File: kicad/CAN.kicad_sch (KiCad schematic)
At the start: 1 part, among them U6 SN65HVD231

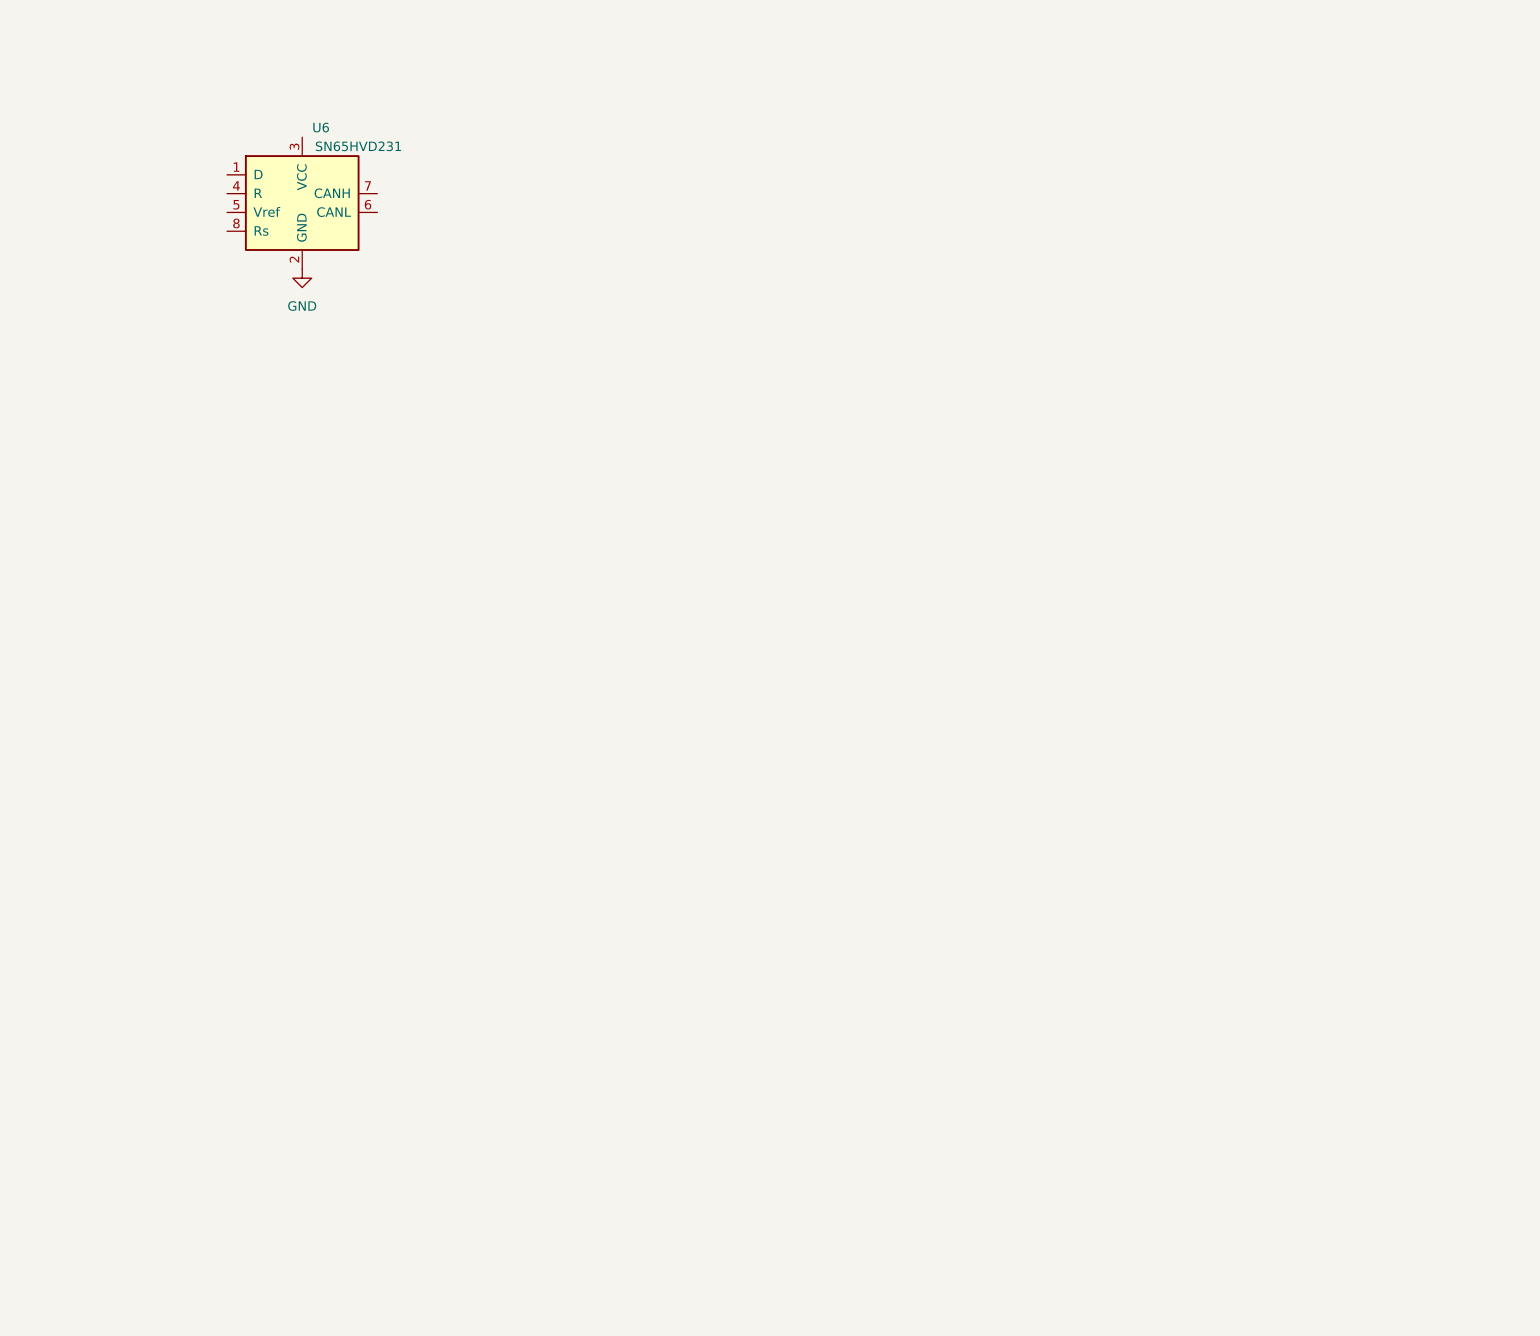
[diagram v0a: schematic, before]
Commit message: WIP
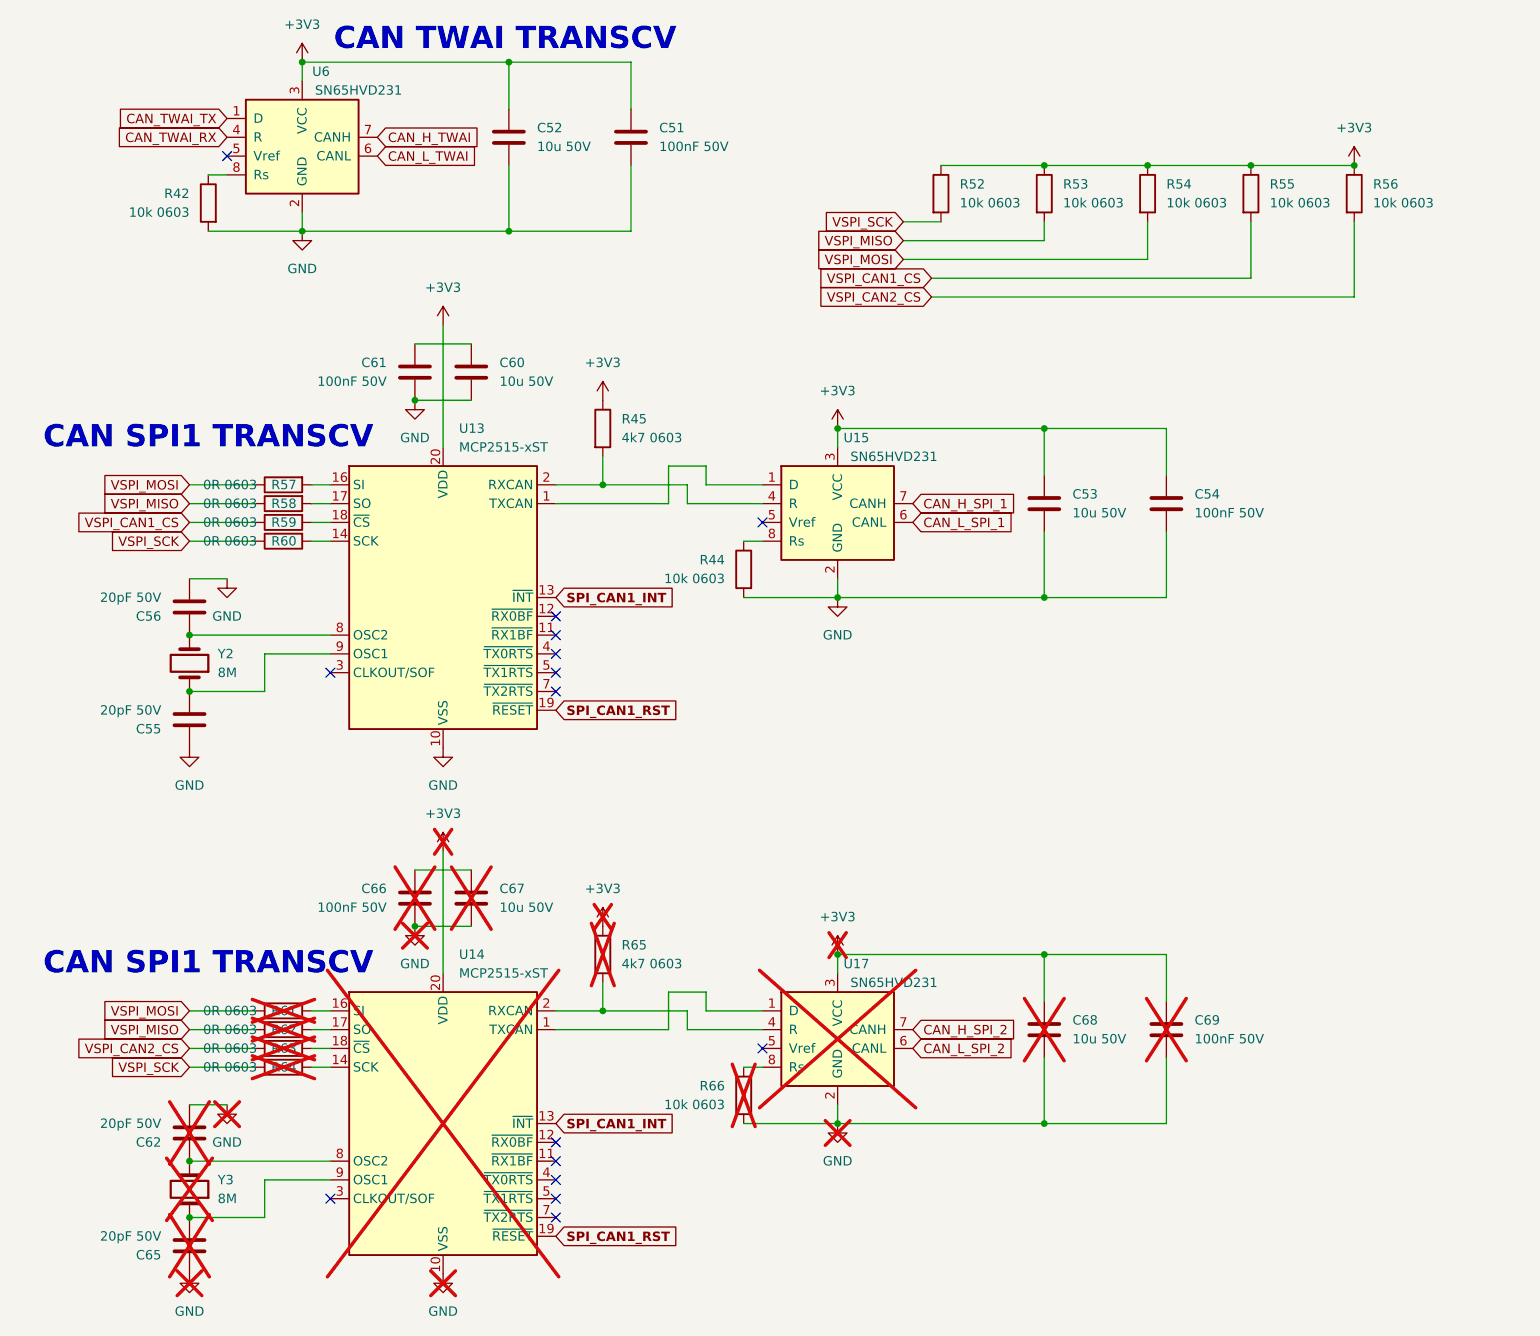
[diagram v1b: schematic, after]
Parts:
- added C51, C54, C61, C66, C69: 100nF 50V, Capacitor_SMD:C_0603_1608Metric, symbol Device:C
- added C52, C53, C60, C67, C68: 10u 50V, Capacitor_SMD:C_1206_3216Metric, symbol Device:C
- added C55, C56, C62, C65: 20pF 50V, Capacitor_SMD:C_0603_1608Metric, symbol Device:C
- added R42, R44, R52, R53, R54, R55, R56, R66: 10k 0603, Resistor_SMD:R_0603_1608Metric, symbol Device:R
- added R45, R65: 4k7 0603, Resistor_SMD:R_0603_1608Metric, symbol Device:R
- added R57, R58, R59, R60, R61, R62, R63, R64: 0R 0603, Resistor_SMD:R_0603_1608Metric, symbol Device:R
- added U13, U14: MCP2515-xST, Package_SO:TSSOP-20_4.4x6.5mm_P0.65mm, symbol Interface_CAN_LIN:MCP2515-xST
- added U15, U17: SN65HVD231, Package_SO:SOIC-8_3.9x4.9mm_P1.27mm, symbol Interface_CAN_LIN:SN65HVD231
- added Y2, Y3: 8M, Crystal:Crystal_HC49-U_Horizontal, symbol Device:Crystal
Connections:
- net GND: now also C51.2, C52.2, C53.2, C54.2, C55.1, C56.2, C60.2, C61.2, C62.2, C65.1, C66.2, C67.2, C68.2, C69.2, R42.2, R44.2, R66.2, U13.10 (VSS), U14.10 (VSS), U15.2 (GND), U17.2 (GND)
- net CAN_TWAI_TX: now reaches U6.1 (D)
- net +3V3: now reaches U6.3 (VCC)
- net +3V3: now also C51.1, C52.1, C53.1, C54.1, C68.1, C69.1, R45.1, R52.1, R53.1, R54.1, R55.1, R56.1, R65.1, U13.20 (VDD), U14.20 (VDD), U15.3 (VCC), U17.3 (VCC)
- net CAN_TWAI_RX: now reaches U6.4 (R)
- net CAN_L_TWAI: now reaches U6.6 (CANL)
- net CAN_H_TWAI: now reaches U6.7 (CANH)
- net at U6.8 (Rs): now also R42.1
- new net: R45.2, U13.2 (RXCAN), U15.4 (R)
- new net: C55.2, U13.9 (OSC1), Y2.1
- new net: R61.2, U14.16 (SI)
- new net: R65.2, U14.2 (RXCAN), U17.4 (R)
- new net: C56.1, U13.8 (OSC2), Y2.2
- new net: C66.1, C67.1
- new net: R44.1, U15.8 (Rs)
- new net: U13.1 (TXCAN), U15.1 (D)
- new net: R60.2, U13.14 (SCK)
- new net: R57.2, U13.16 (SI)
- new net: R58.2, U13.17 (SO)
- new net: R59.2, U13.18 (~{CS})
- new net: R66.1, U17.8 (Rs)
- new net: U14.1 (TXCAN), U17.1 (D)
- new net: R64.2, U14.14 (SCK)
- new net: R62.2, U14.17 (SO)
- new net: R63.2, U14.18 (~{CS})
- new net: C62.1, U14.8 (OSC2), Y3.2
- new net: C65.2, U14.9 (OSC1), Y3.1
- new net: C60.1, C61.1
- new net CAN_H_SPI_1: U15.7 (CANH)
- new net CAN_H_SPI_2: U17.7 (CANH)
- new net CAN_L_SPI_1: U15.6 (CANL)
- new net CAN_L_SPI_2: U17.6 (CANL)
- new net SPI_CAN1_INT: U13.13 (~{INT}), U14.13 (~{INT})
- new net SPI_CAN1_RST: U13.19 (~{RESET}), U14.19 (~{RESET})
- new net VSPI_CAN1_CS: R55.2, R59.1
- new net VSPI_CAN2_CS: R56.2, R63.1
- new net VSPI_MISO: R53.2, R58.1, R62.1
- new net VSPI_MOSI: R54.2, R57.1, R61.1
- new net VSPI_SCK: R52.2, R60.1, R64.1
- no-connect marks 0 -> 15
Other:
- note added: "CAN SPI1 TRANSCV"
- note added: "CAN TWAI TRANSCV"
- moved on the sheet: U6

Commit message: sch done-ish
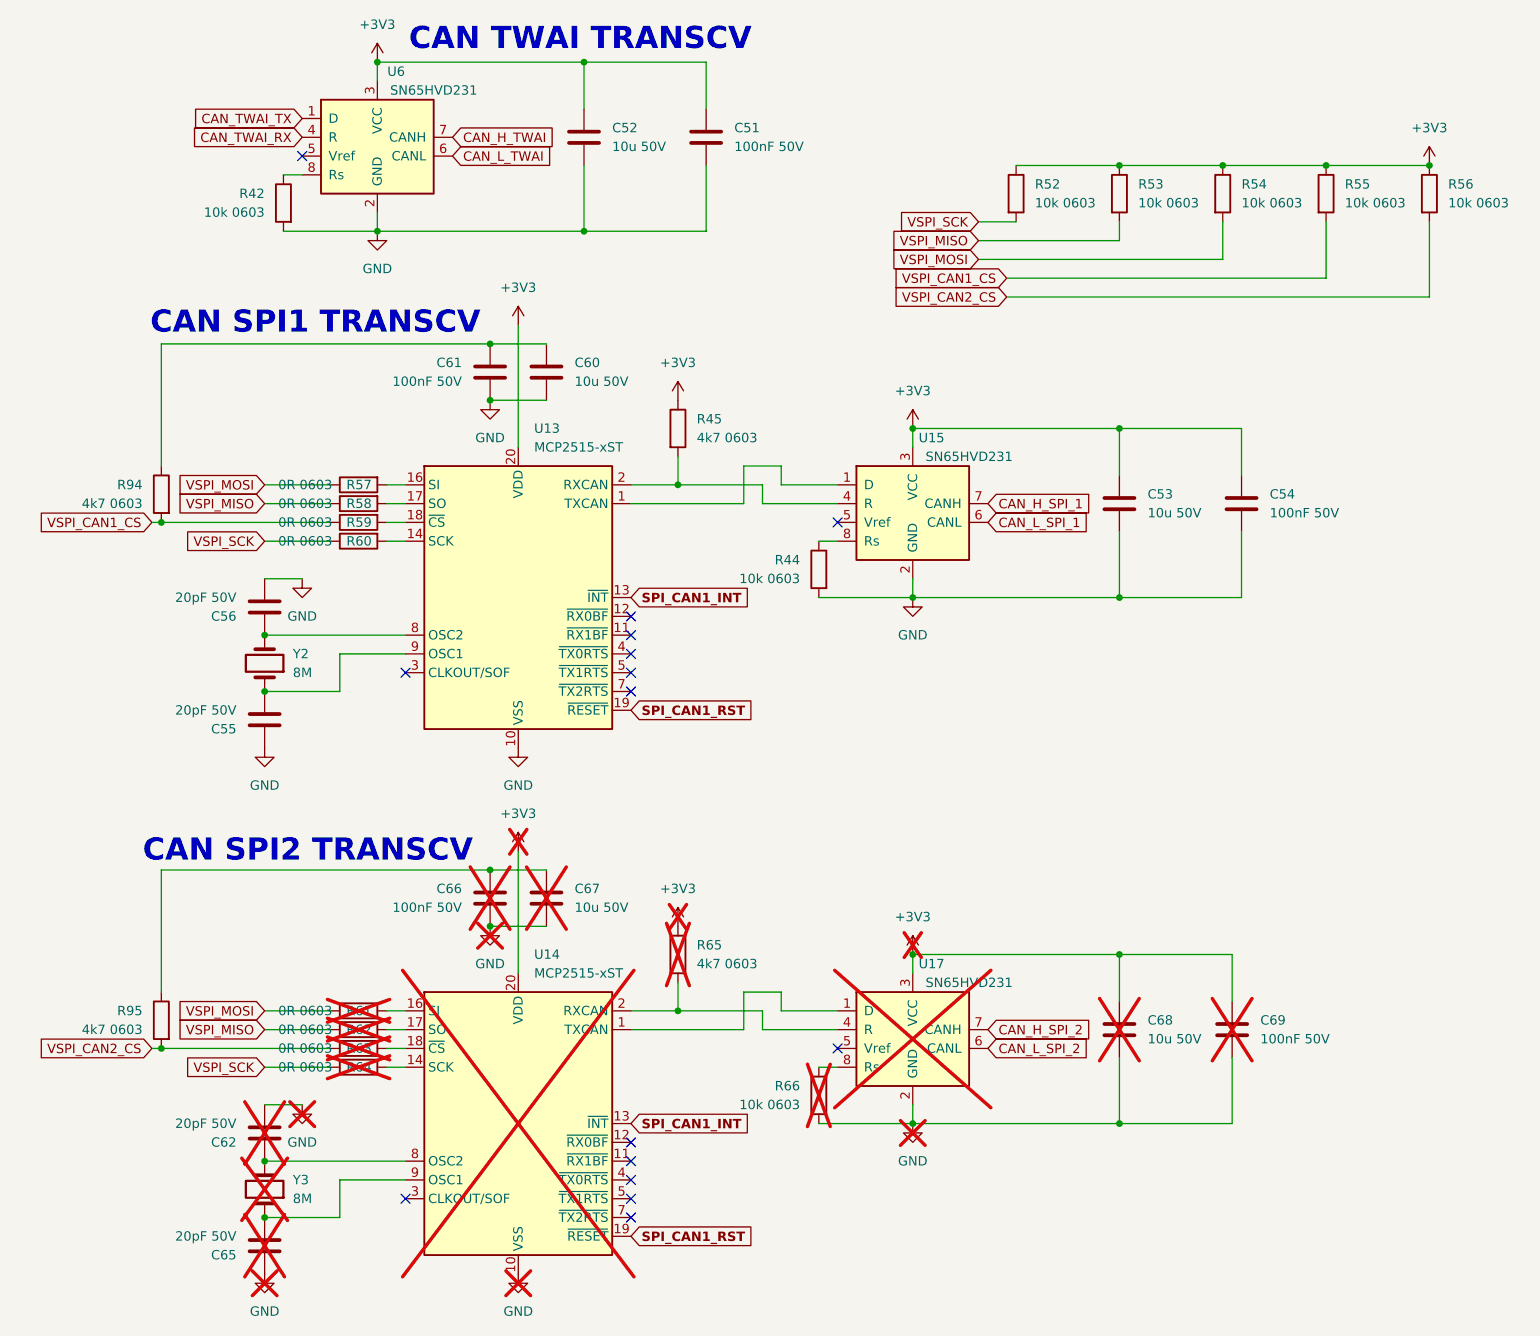
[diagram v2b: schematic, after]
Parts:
- added R94, R95: 4k7 0603, Resistor_SMD:R_0603_1608Metric, symbol Device:R
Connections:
- net VSPI_CAN1_CS: now also R94.2
- net VSPI_CAN2_CS: now also R95.2
- net at C66.1, C67.1: now also R95.1
- net at C60.1, C61.1: now also R94.1
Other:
- note added: "CAN SPI2 TRANSCV"
- company: (none) -> ©CC-BY-NC
- title: (none) -> VehicleMan
- moved on the sheet: C51, C52, C53, C54, C55, C56, C60, C61, C62, C65, C66, C67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
